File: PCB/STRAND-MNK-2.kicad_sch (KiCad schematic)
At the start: 4 parts

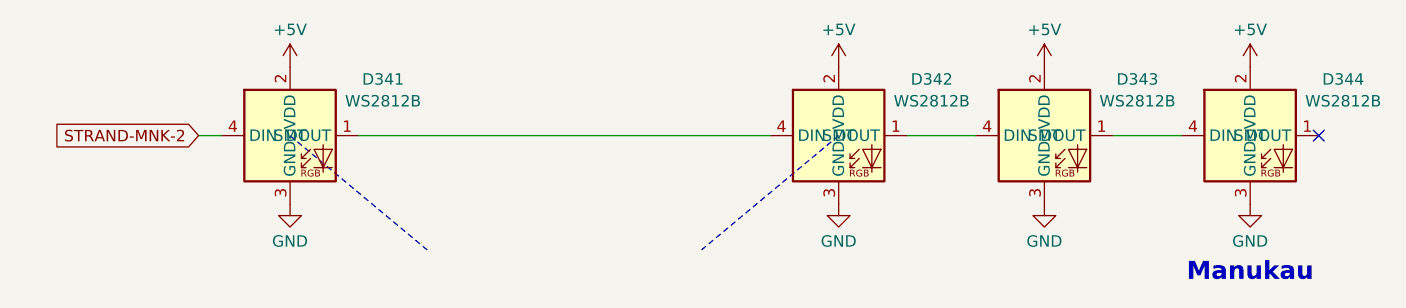
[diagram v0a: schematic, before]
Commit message: V1.1.0 PCB
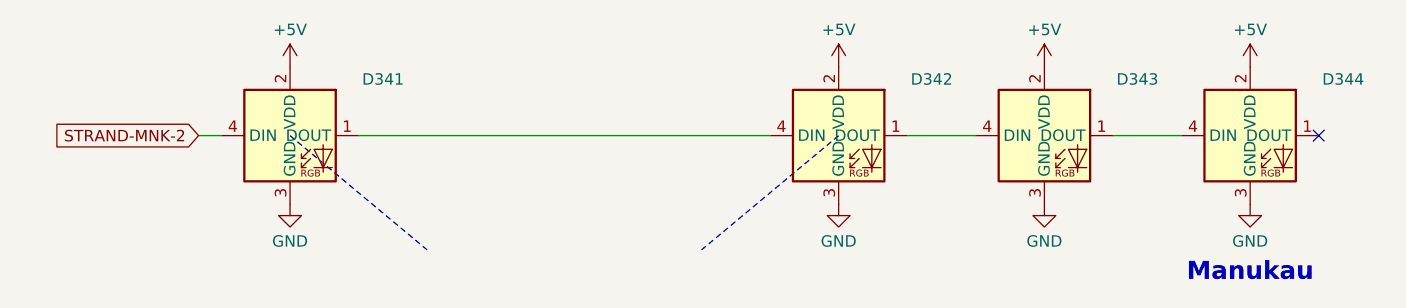
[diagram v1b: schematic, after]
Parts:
- D341, D342, D343, D344: value WS2812B -> XL-1615RGBC-WS2812B-S; LCSC C5349954 -> C41413180; Manufacturer XINGLIGHT -> (none); Part XL-1615RGBC-WS2812B -> (none); Process SMT -> (none)
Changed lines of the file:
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@@
 	(title_block
 		(title "Auckland Train Network Live Map")
-		(date "2025-04-26")
-		(rev "1")
+		(date "2025-06-23")
+		(rev "1.1.0")
 		(company "Kea Studios")
 		(comment 1 "©Chris Dirks")
@@
 			)
 		)
-		(property "Value" "WS2812B"
+		(property "Value" "XL-1615RGBC-WS2812B-S"
 			(at 134.7976 24.1177 0)
 			(effects
@@
 					(size 1.27 1.27)
 				)
+				(hide yes)
 			)
 		)
@@
 			)
 		)
-		(property "LCSC" "C5349954"
+		(property "LCSC" "C41413180"
 			(at 124.46 27.94 0)
 			(effects
@@
 			)
 		)
-		(property "Part" "XL-1615RGBC-WS2812B"
+		(property "Circuits" ""
 			(at 124.46 27.94 0)
 			(effects
@@
 			)
 		)
-		(property "Manufacturer" "XINGLIGHT"
+		(property "Current Rating" ""
 			(at 124.46 27.94 0)
 			(effects
@@
 			)
 		)
-		(property "PartID" ""
+		(property "DC Resistance" ""
 			(at 124.46 27.94 0)
 			(effects
@@
 					(size 1.27 1.27)
 				)
-			)
-		)
-		(property "Process" "SMT"
+				(hide yes)
+			)
+		)
+		(property "Impedance @ Frequency" ""
 			(at 124.46 27.94 0)
 			(effects
@@
 					(size 1.27 1.27)
 				)
+				(hide yes)
 			)
 		)
@@
 			)
 		)
-		(property "Value" "WS2812B"
+		(property "Value" "XL-1615RGBC-WS2812B-S"
 			(at 157.6576 24.1177 0)
 			(effects
@@
 					(size 1.27 1.27)
 				)
+				(hide yes)
 			)
 		)
@@
 			)
 		)
-		(property "LCSC" "C5349954"
+		(property "LCSC" "C41413180"
 			(at 147.32 27.94 0)
 			(effects
@@
 			)
 		)
-		(property "Part" "XL-1615RGBC-WS2812B"
+		(property "Circuits" ""
 			(at 147.32 27.94 0)
 			(effects
@@
 			)
 		)
-		(property "Manufacturer" "XINGLIGHT"
+		(property "Current Rating" ""
 			(at 147.32 27.94 0)
 			(effects
@@
 			)
 		)
-		(property "PartID" ""
+		(property "DC Resistance" ""
 			(at 147.32 27.94 0)
 			(effects
@@
 					(size 1.27 1.27)
 				)
-			)
-		)
-		(property "Process" "SMT"
+				(hide yes)
+			)
+		)
+		(property "Impedance @ Frequency" ""
 			(at 147.32 27.94 0)
 			(effects
@@
 					(size 1.27 1.27)
 				)
+				(hide yes)
 			)
 		)
@@
 			)
 		)
-		(property "Value" "WS2812B"
+		(property "Value" "XL-1615RGBC-WS2812B-S"
 			(at 111.9376 24.1177 0)
 			(effects
@@
 					(size 1.27 1.27)
 				)
+				(hide yes)
 			)
 		)
@@
 			)
 		)
-		(property "LCSC" "C5349954"
+		(property "LCSC" "C41413180"
 			(at 101.6 27.94 0)
 			(effects
@@
 			)
 		)
-		(property "Part" "XL-1615RGBC-WS2812B"
+		(property "Circuits" ""
 			(at 101.6 27.94 0)
 			(effects
@@
 			)
 		)
-		(property "Manufacturer" "XINGLIGHT"
+		(property "Current Rating" ""
 			(at 101.6 27.94 0)
 			(effects
@@
 			)
 		)
-		(property "PartID" ""
+		(property "DC Resistance" ""
 			(at 101.6 27.94 0)
 			(effects
@@
 					(size 1.27 1.27)
 				)
-			)
-		)
-		(property "Process" "SMT"
+				(hide yes)
+			)
+		)
+		(property "Impedance @ Frequency" ""
 			(at 101.6 27.94 0)
 			(effects
@@
 					(size 1.27 1.27)
 				)
+				(hide yes)
 			)
 		)
@@
 			)
 		)
-		(property "Value" "WS2812B"
+		(property "Value" "XL-1615RGBC-WS2812B-S"
 			(at 50.9776 24.1177 0)
 			(effects
@@
 					(size 1.27 1.27)
 				)
+				(hide yes)
 			)
 		)
@@
 			)
 		)
-		(property "LCSC" "C5349954"
+		(property "LCSC" "C41413180"
 			(at 40.64 27.94 0)
 			(effects
@@
 			)
 		)
-		(property "Part" "XL-1615RGBC-WS2812B"
+		(property "Circuits" ""
 			(at 40.64 27.94 0)
 			(effects
@@
 			)
 		)
-		(property "Manufacturer" "XINGLIGHT"
+		(property "Current Rating" ""
 			(at 40.64 27.94 0)
 			(effects
@@
 			)
 		)
-		(property "PartID" ""
+		(property "DC Resistance" ""
 			(at 40.64 27.94 0)
 			(effects
@@
 					(size 1.27 1.27)
 				)
-			)
-		)
-		(property "Process" "SMT"
+				(hide yes)
+			)
+		)
+		(property "Impedance @ Frequency" ""
 			(at 40.64 27.94 0)
 			(effects
@@
 					(size 1.27 1.27)
 				)
-			)
-		)
+				(hide yes)
+			)
+		)
